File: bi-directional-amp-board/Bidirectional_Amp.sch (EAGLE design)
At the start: 130 parts, among them J1 73415-2061, J10 73415-2061, J11 73415-2061, J12 73415-2061, J2 73415-2061, J3 22-23-2071, J4 73415-2061, J5 73415-2061, J6 73415-2061, J7 73415-2061, J8 73415-2061, J9 22-23-2031, U1 LTC5536, U10 NC7S32M5X, U11 SN74LV1T34DBVR, U2 LTC6994-1, U3 LTC6994-1, U4 QPC1022, U5 NC7S04M5, U6 TQP9111, U7 TQP3M9035, U8 QPC1022, U9 LTC3428EDDPBF

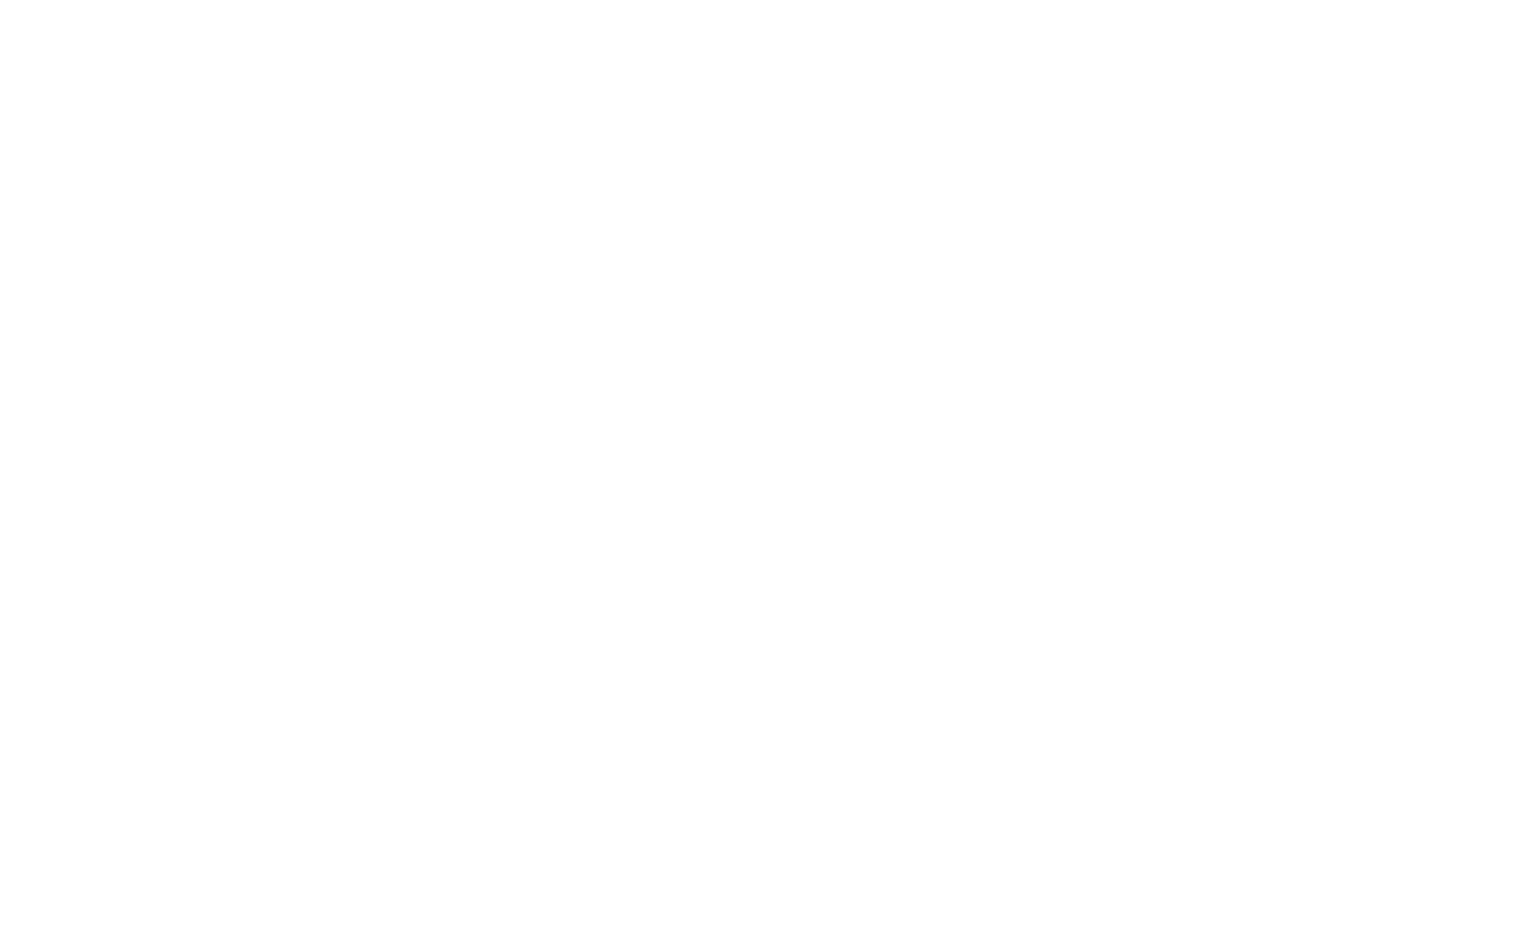
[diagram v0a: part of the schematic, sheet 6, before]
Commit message: lots of progress on wifi board
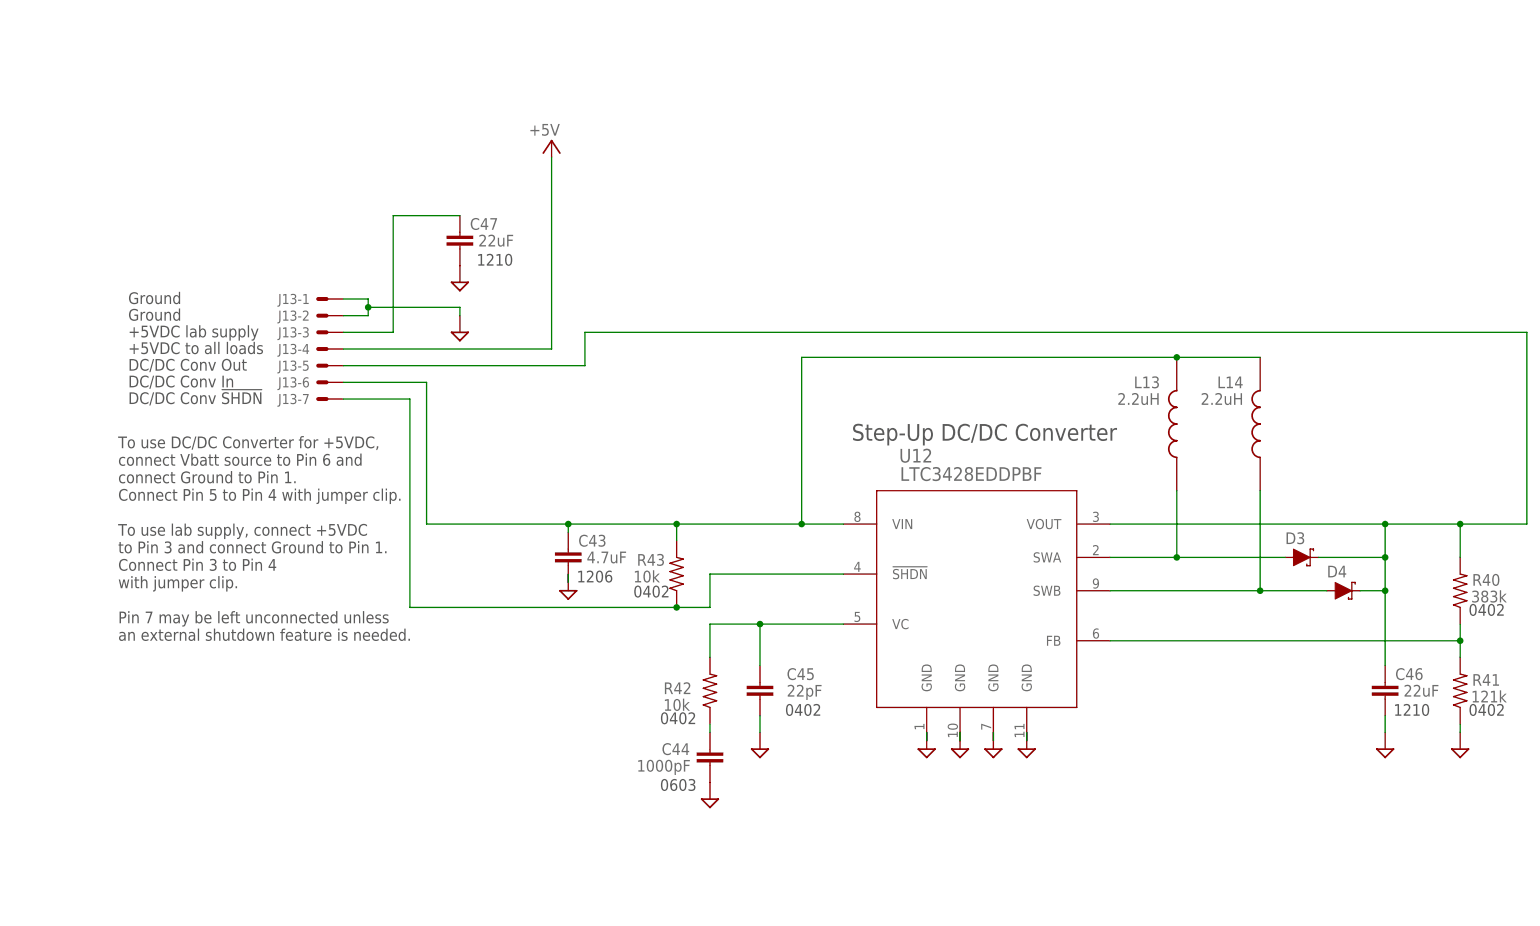
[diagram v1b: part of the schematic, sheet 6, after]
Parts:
- added C43: 4.7uF, rcl:C-EUC1206
- added C44: 1000pF, rcl:C-EUC0603
- added C45: 22pF, rcl:C-EUC0402
- added C46, C47: 22uF, rcl:C-EUC1210
- added D3, D4: DIODE-SCHOTTKY-PMEG4005EJ, SparkFun-DiscreteSemi:DIODE-SCHOTTKY-PMEG4005EJ
- added J13: 22-23-2071, 22-23-2071:22-23-2071
- added L13, L14: 2.2uH, SamacSys_Parts:XFL4020-222MEB
- added R40: 383k, oresat-rcl:R-US_0402-B-NOSILK
- added R41: 121k, oresat-rcl:R-US_0402-B-NOSILK
- added R42, R43: 10k, oresat-rcl:R-US_0402-B-NOSILK
- added U12: LTC3428EDDPBF, LTC3428:LTC3428EDDPBF
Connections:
- new net FB1: R40.1, R41.2, U12.FB
- new net N$23: C44.1, R42.1
- new net N$36: C47.1, J13-3.S
- new net SHDN1: J13-7.S, R43.1, U12.!SHDN
- new net SWA1: D3.A, L13.1, U12.SWA
- new net SWB1: D4.A, L14.1, U12.SWB
- new net VC1: C45.1, R42.2, U12.VC
- new net VIN1: C43.1, J13-6.S, L13.2, L14.2, R43.2, U12.VIN
- new net VOUT1: C46.1, D3.C, D4.C, J13-5.S, R40.2, U12.VOUT
- net +5V: now also J13-4.S
- net GND: now also C43.2, C44.2, C45.2, C46.2, C47.2, J13-1.S, J13-2.S, R41.1, U12.GND@1, U12.GND@10, U12.GND@11, U12.GND@7
